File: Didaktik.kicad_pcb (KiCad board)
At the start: 2 copper layers, 209.6 x 76.2 mm, 129 parts, among them J1 Conn_01x04_MountingPin, J2 AVR-ISP-6, J3 Conn_01x03, Q1 2N2222, SW1 SW_Push_45deg, SW10 SW_Push_45deg, SW11 SW_Push_45deg, SW12 SW_Push_45deg, SW13 SW_Push_45deg, SW14 SW_Push_45deg, SW15 SW_Push_45deg, SW16 SW_Push_45deg, SW17 SW_Push_45deg, SW18 SW_Push_45deg, SW19 SW_Push_45deg, SW2 SW_Push_45deg, SW20 SW_Push_45deg, SW21 SW_Push_45deg, SW22 SW_Push_45deg, SW23 SW_Push_45deg, SW24 SW_Push_45deg, SW25 SW_Push_45deg, SW26 SW_Push_45deg, SW27 SW_Push_45deg, SW28 SW_Push_45deg, SW29 SW_Push_45deg, SW3 SW_Push_45deg, SW30 SW_Push_45deg, SW31 SW_Push_45deg, SW31a1 SW_Push_45deg, SW32 SW_Push_45deg, SW32a1 SW_Push_45deg, SW33 SW_Push_45deg, SW33a1 SW_Push_45deg, SW34 SW_Push_45deg, SW34a1 SW_Push_45deg, SW34b1 SW_Push_45deg, SW35 SW_Push_45deg, SW35a1 SW_Push_45deg, SW35b1 SW_Push_45deg, SW35c1 SW_Push_45deg, SW36 SW_Push_45deg, SW36a1 SW_Push_45deg, SW36b1 SW_Push_45deg, SW36c1 SW_Push_45deg, SW37 SW_Push_45deg, SW37a1 SW_Push_45deg, SW37b1 SW_Push_45deg, SW38 SW_Push_45deg, SW38a1 SW_Push_45deg, SW39 SW_Push_45deg, SW39a1 SW_Push_45deg, SW4 SW_Push_45deg, SW40 SW_Push_45deg, SW40a1 SW_Push_45deg, SW41 RotaryEncoder_Switch, SW42 RotaryEncoder_Switch, SW5 SW_Push_45deg, SW6 SW_Push_45deg, SW7 SW_Push_45deg, SW8 SW_Push_45deg, SW9 SW_Push_45deg, U1 ATmega32U4-M, Y1 Crystal_GND24_Small

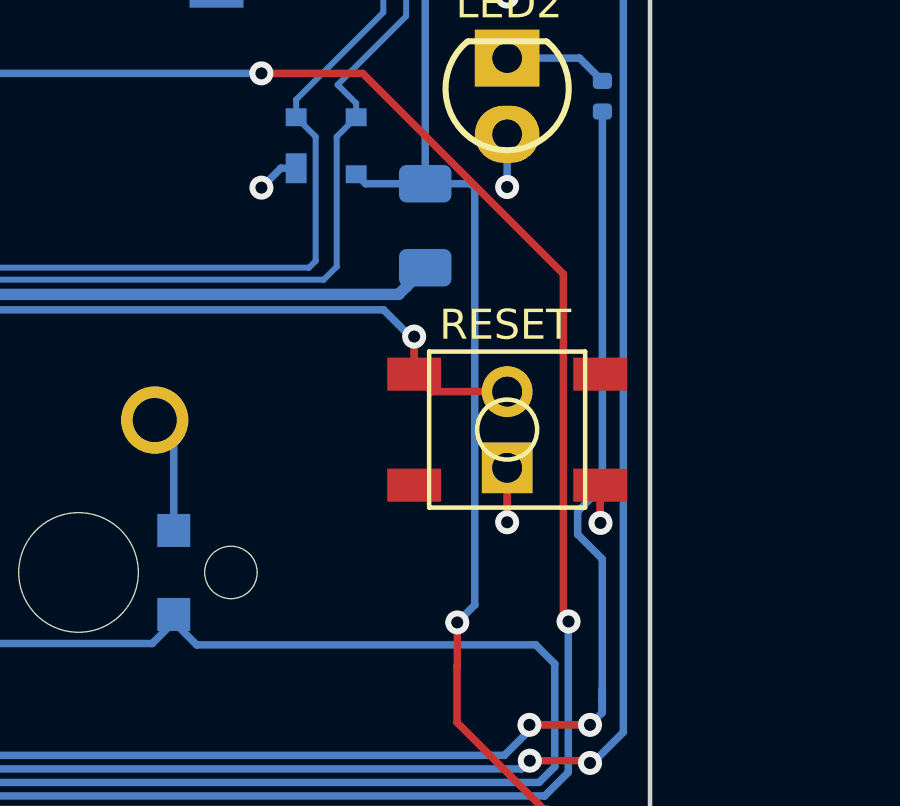
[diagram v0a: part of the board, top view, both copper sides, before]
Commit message: added STEM project WIP
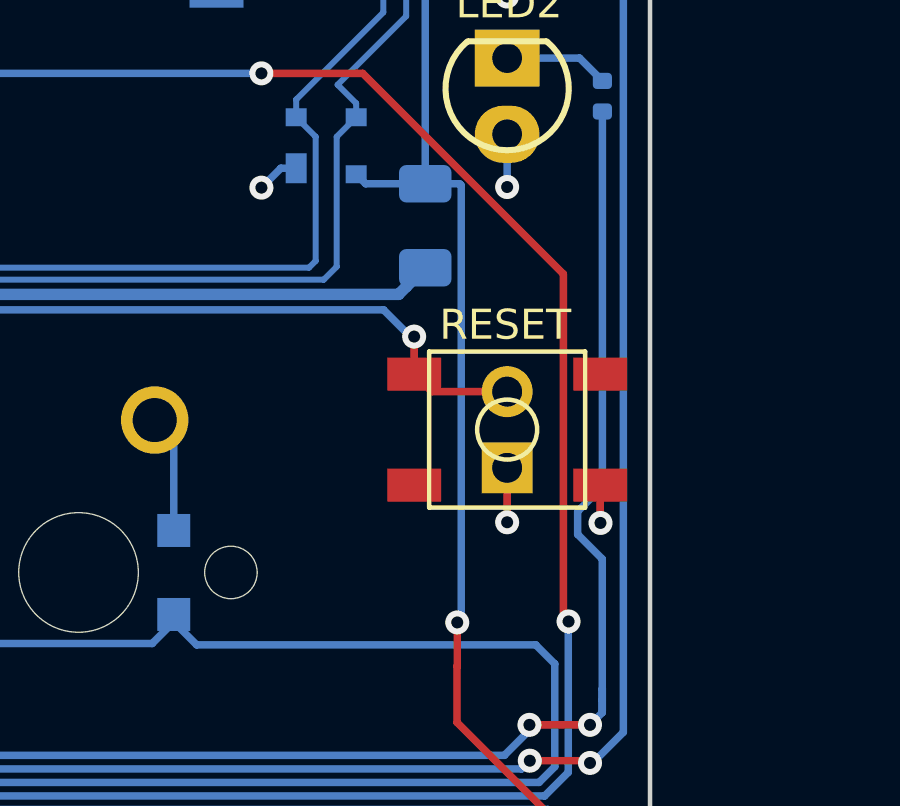
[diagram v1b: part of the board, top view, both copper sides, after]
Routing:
- net VCC: track 261.1 -> 260.5 mm
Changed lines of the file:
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@@
   (segment (start 231.822 47.368) (end 231.505 47.051) (width 0.25) (layer "B.Cu") (net 62))
   (segment (start 225.425 82.5405) (end 225.425 82.55) (width 0.25) (layer "B.Cu") (net 62))
-  (segment (start 233.807 47.368) (end 235.328 47.368) (width 0.25) (layer "B.Cu") (net 62))
   (segment (start 229.625 35.975) (end 229.6735 35.975) (width 0.25) (layer "B.Cu") (net 62))
-  (segment (start 235.331 47.371) (end 235.458 47.498) (width 0.25) (layer "B.Cu") (net 62))
   (segment (start 229.625 39.2875) (end 229.625 35.975) (width 0.25) (layer "B.Cu") (net 62))
   (segment (start 225.425 84.4395) (end 225.1505 84.165) (width 0.25) (layer "B.Cu") (net 62))
   (segment (start 62.253 89.789) (end 62.253 84.559) (width 0.25) (layer "B.Cu") (net 62))
+  (segment (start 233.807 47.368) (end 234.95 47.368) (width 0.25) (layer "B.Cu") (net 62))
   (segment (start 225.425 82.55) (end 225.679 82.804) (width 0.25) (layer "B.Cu") (net 62))
-  (segment (start 235.458 61.407655) (end 235.458 47.498) (width 0.25) (layer "B.Cu") (net 62))
-  (segment (start 234.874569 61.991086) (end 235.458 61.407655) (width 0.25) (layer "B.Cu") (net 62))
+  (segment (start 234.95 47.368) (end 235.007 47.425) (width 0.25) (layer "B.Cu") (net 62))
+  (segment (start 235.007 61.858655) (end 234.874569 61.991086) (width 0.25) (layer "B.Cu") (net 62))
   (segment (start 225.1505 84.165) (end 62.829 84.165) (width 0.25) (layer "B.Cu") (net 62))
   (segment (start 62.647 84.165) (end 62.829 84.165) (width 0.25) (layer "B.Cu") (net 62))
   (segment (start 229.9375 39.6) (end 229.625 39.2875) (width 0.25) (layer "B.Cu") (net 62))
-  (segment (start 235.328 47.368) (end 235.331 47.371) (width 0.25) (layer "B.Cu") (net 62))
   (segment (start 237.363 82.804) (end 237.617 82.55) (width 0.25) (layer "B.Cu") (net 62))
   (segment (start 229.9615 35.687) (end 233.1365 35.687) (width 0.25) (layer "B.Cu") (net 62))
@@
   (segment (start 225.679 82.804) (end 237.363 82.804) (width 0.25) (layer "B.Cu") (net 62))
   (segment (start 229.6735 35.975) (end 229.9615 35.687) (width 0.25) (layer "B.Cu") (net 62))
+  (segment (start 235.007 47.425) (end 235.007 61.858655) (width 0.25) (layer "B.Cu") (net 62))
   (segment (start 233.807 47.368) (end 233.807 36.3575) (width 0.25) (layer "B.Cu") (net 62))
   (segment (start 62.253 84.559) (end 62.647 84.165) (width 0.25) (layer "B.Cu") (net 62))
